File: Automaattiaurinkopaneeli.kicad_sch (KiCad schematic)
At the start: 17 parts, among them J1 Conn_02x04_Row_Letter_Last, J10 Conn_01x08_Socket, J2 Conn_02x01, J3 Conn_01x02_Pin, J4 Conn_01x03_Pin, J5 Conn_01x03_Pin, J6 Conn_01x05_Pin, J7 Barrel_Jack_Switch, J8 Conn_01x02_Pin, J9 Conn_01x08_Socket, U1 ESP32-WROOM-32D, U2 ACS712xLCTR-20A, U3 LF33_TO220

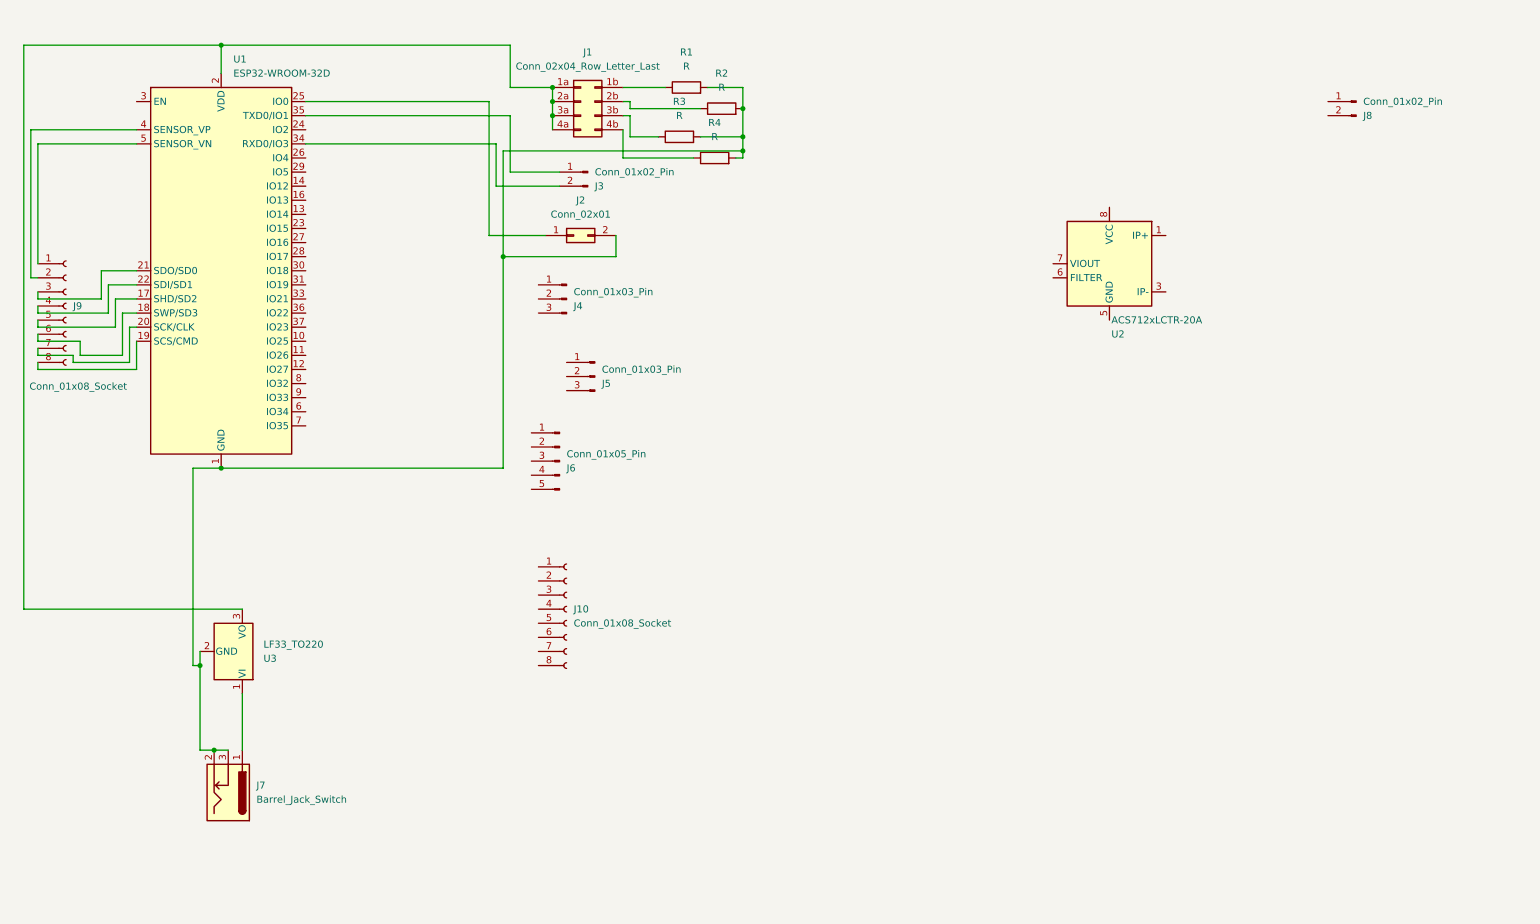
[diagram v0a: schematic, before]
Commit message: end of day and final desing
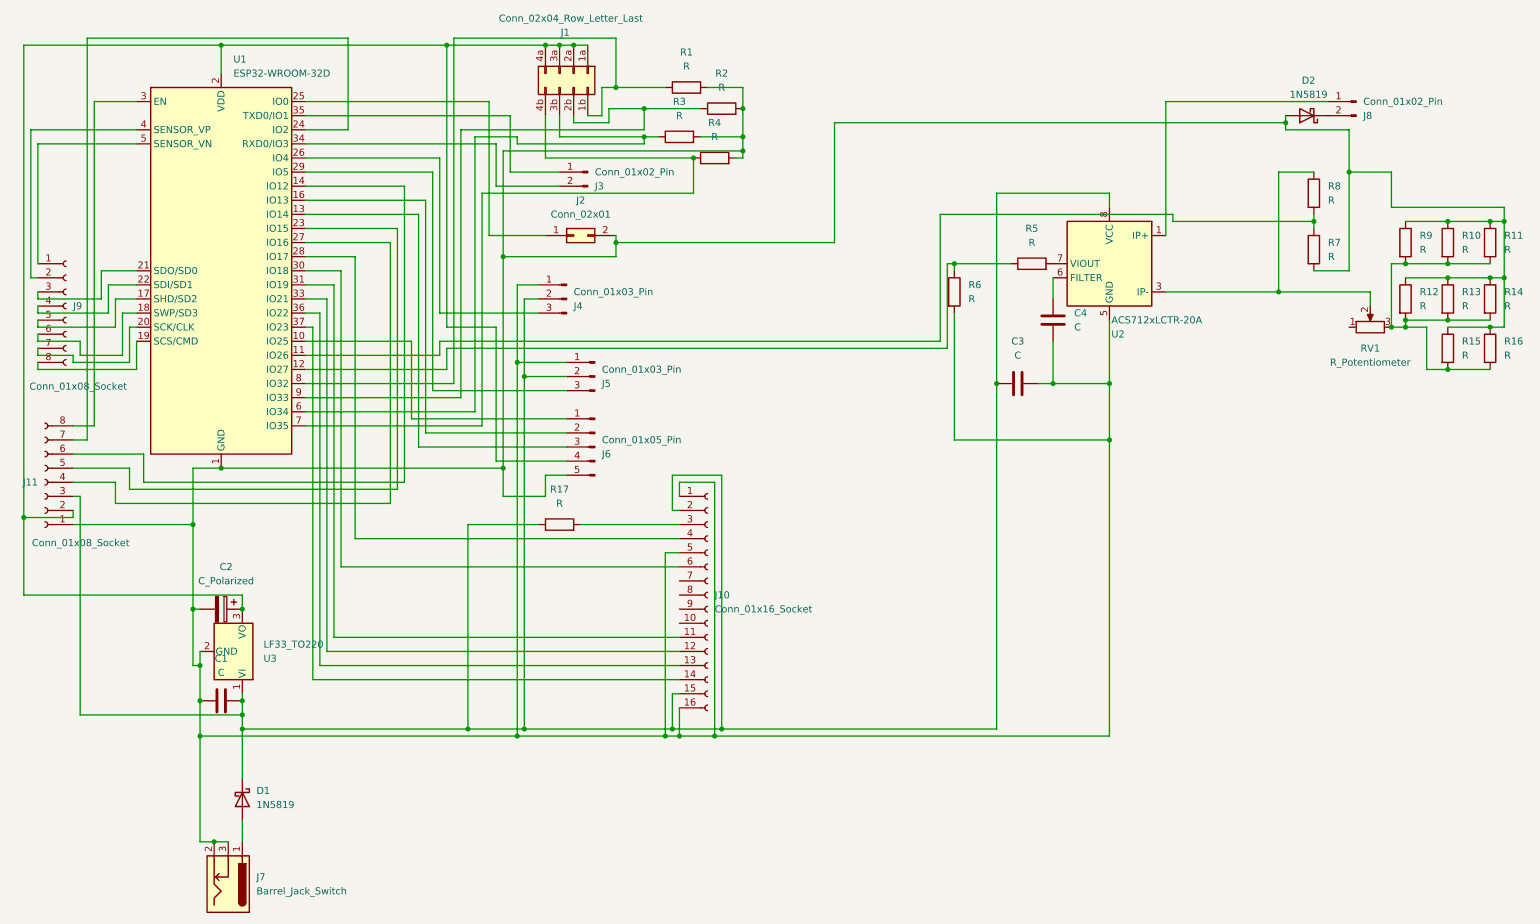
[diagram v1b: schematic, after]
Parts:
- removed J10: Conn_01x08_Socket, Connector_PinSocket_2.54mm:PinSocket_1x08_P2.54mm_Vertical, symbol Connector:Conn_01x08_Socket
- added C1: C, Capacitor_THT:C_Rect_L4.6mm_W4.6mm_P2.50mm_MKS02_FKP02, symbol Device:C
- added C2: C_Polarized, Capacitor_THT:CP_Radial_D5.0mm_P2.00mm, symbol Device:C_Polarized
- added C3, C4: C, Capacitor_THT:C_Disc_D10.0mm_W2.5mm_P5.00mm, symbol Device:C
- added D1, D2: 1N5819, Diode_THT:D_DO-41_SOD81_P10.16mm_Horizontal, symbol Diode:1N5819
- added J10: Conn_01x16_Socket, Connector_PinSocket_2.54mm:PinSocket_1x16_P2.54mm_Vertical, symbol Connector:Conn_01x16_Socket
- added J11: Conn_01x08_Socket, Connector_PinSocket_2.54mm:PinSocket_1x08_P2.54mm_Vertical, symbol Connector:Conn_01x08_Socket
- added R10, R11, R12, R13, R14, R15, R16, R17, R5, R6, R7, R8, R9: R, Resistor_THT:R_Axial_DIN0207_L6.3mm_D2.5mm_P10.16mm_Horizontal, symbol Device:R
- added RV1: R_Potentiometer, Potentiometer_THT:Potentiometer_Vishay_148-149_Single_Horizontal, symbol Device:R_Potentiometer
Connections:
- net at J6.1 (Pin_1): now also U1.10 (IO25)
- net at J6.2 (Pin_2): now also U1.16 (IO13)
- net at J6.3 (Pin_3): now also U1.13 (IO14)
- net at J6.4 (Pin_4): now also J1.1a (Pin_1a), J1.2a (Pin_2a), J1.3a (Pin_3a), J1.4a (Pin_4a), U1.2 (VDD), U3.3 (VO), C2.1, J11.2 (Pin_2)
- net at J6.5 (Pin_5): now also J2.2 (Pin_2), J4.1 (Pin_1), J5.1 (Pin_1), J7.2, J7.3, R1.2, R2.2, R3.2, R4.2, U1.1 (GND), U1.15 (GND), U1.38 (GND), U1.39 (GND), U2.5 (GND), U3.2 (GND), C1.1, C2.2, C3.2, C4.2, D2.2 (A), J10.1 (Pin_1), J10.16 (Pin_16), J10.5 (Pin_5), J11.1 (Pin_1), R10.1, R11.1, R12.1, R13.1, R14.1, R15.1, R16.1, R6.2, R7.2, R9.1
- net at J5.2 (Pin_2): now also J4.2 (Pin_2), U2.8 (VCC), U3.1 (VI), C1.2, C3.1, D1.1 (K), J10.15 (Pin_15), J10.2 (Pin_2), J11.3 (Pin_3), R17.1
- net at J5.3 (Pin_3): now also U1.29 (IO5)
- net at J1.1b (Pin_1b), R1.1: now also U1.8 (IO32)
- net at J1.2b (Pin_2b), R2.1: now also U1.9 (IO33)
- net at J1.3b (Pin_3b), R3.1: now also U1.6 (IO34)
- net at J1.4b (Pin_4b), R4.1: now also U1.7 (IO35)
- net at J8.1 (Pin_1): now also U2.1 (IP+), U2.2 (IP+)
- net at J8.2 (Pin_2): now also D2.1 (K)
- net at U1.11 (IO26): now also R7.1, R8.2
- net at U1.12 (IO27): now also R5.1, R6.1
- net at U1.14 (IO12): now also J11.6 (Pin_6)
- net at U1.23 (IO15): now also J11.5 (Pin_5)
- net at U1.24 (IO2): now also J11.7 (Pin_7)
- net at U1.26 (IO4): now also J4.3 (Pin_3)
- net at U1.27 (IO16): now also J11.4 (Pin_4)
- net at U1.28 (IO17): now also J10.4 (Pin_4)
- net at U1.3 (EN): now also J11.8 (Pin_8)
- net at U1.30 (IO18): now also J10.6 (Pin_6)
- net at U1.31 (IO19): now also J10.11 (Pin_11)
- net at U1.33 (IO21): now also J10.12 (Pin_12)
- net at U1.36 (IO22): now also J10.13 (Pin_13)
- net at U1.37 (IO23): now also J10.14 (Pin_14)
- net at U2.3 (IP-), U2.4 (IP-): now also R8.1, RV1.2
- net at U2.6 (FILTER): now also C4.1
- net at U2.7 (VIOUT): now also R5.2
- net at J7.1: now also D1.2 (A); no longer U3.1 (VI)
- new net: J10.3 (Pin_3), R17.2
- new net: R10.2, R11.2, R12.2, R13.2, R14.2, R15.2, R16.2, R9.2, RV1.3
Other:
- moved on the sheet: J1, J6, J7
